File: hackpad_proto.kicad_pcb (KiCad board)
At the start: 2 copper layers, 110 x 97 mm, 40 parts, among them J1 Conn_01x04, SW1 SW_Push, SW10 SW_Push, SW11 SW_Push, SW12 SW_Push, SW13 RotaryEncoder_Switch, SW2 SW_Push, SW3 SW_Push, SW4 SW_Push, SW5 SW_Push, SW6 SW_Push, SW7 SW_Push, SW8 SW_Push, SW9 SW_Push, U1 XIAO-RP2040-DIP

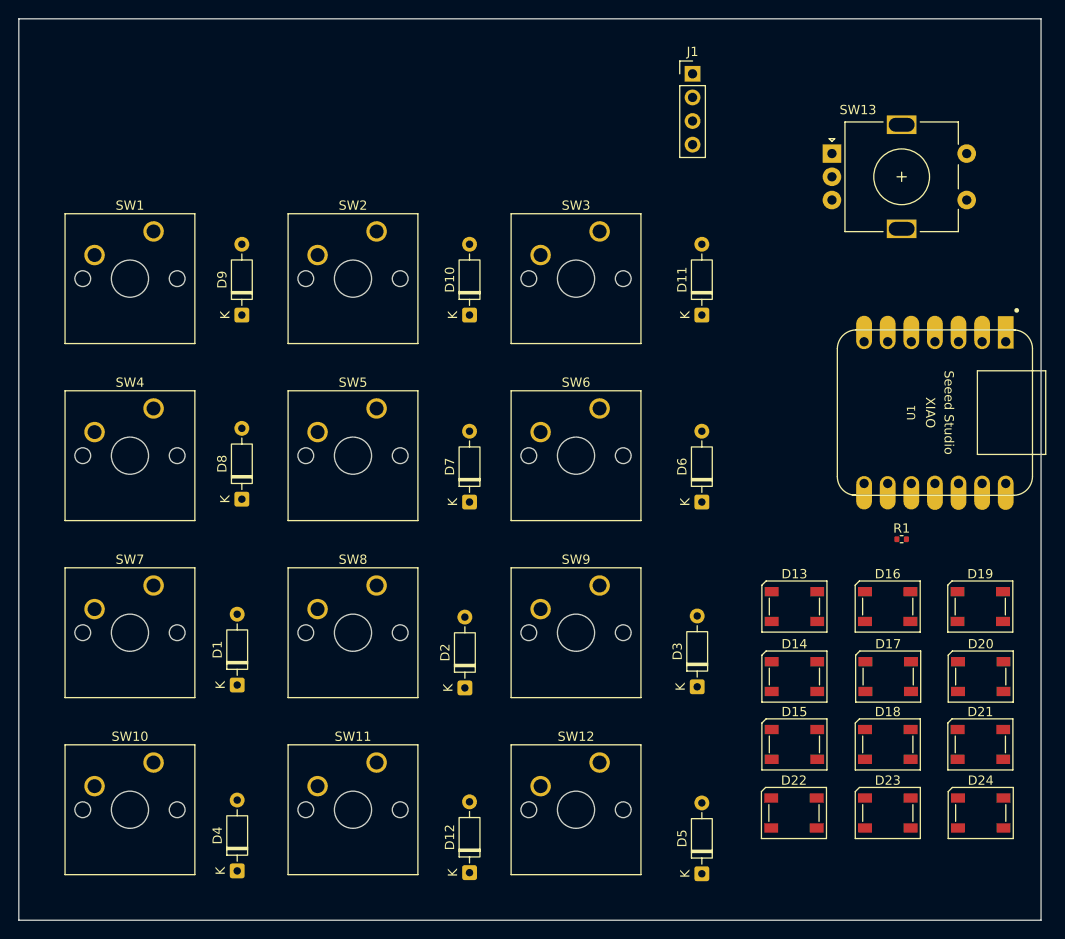
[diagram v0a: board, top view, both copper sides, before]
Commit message: Updated NostPad hardware design layout
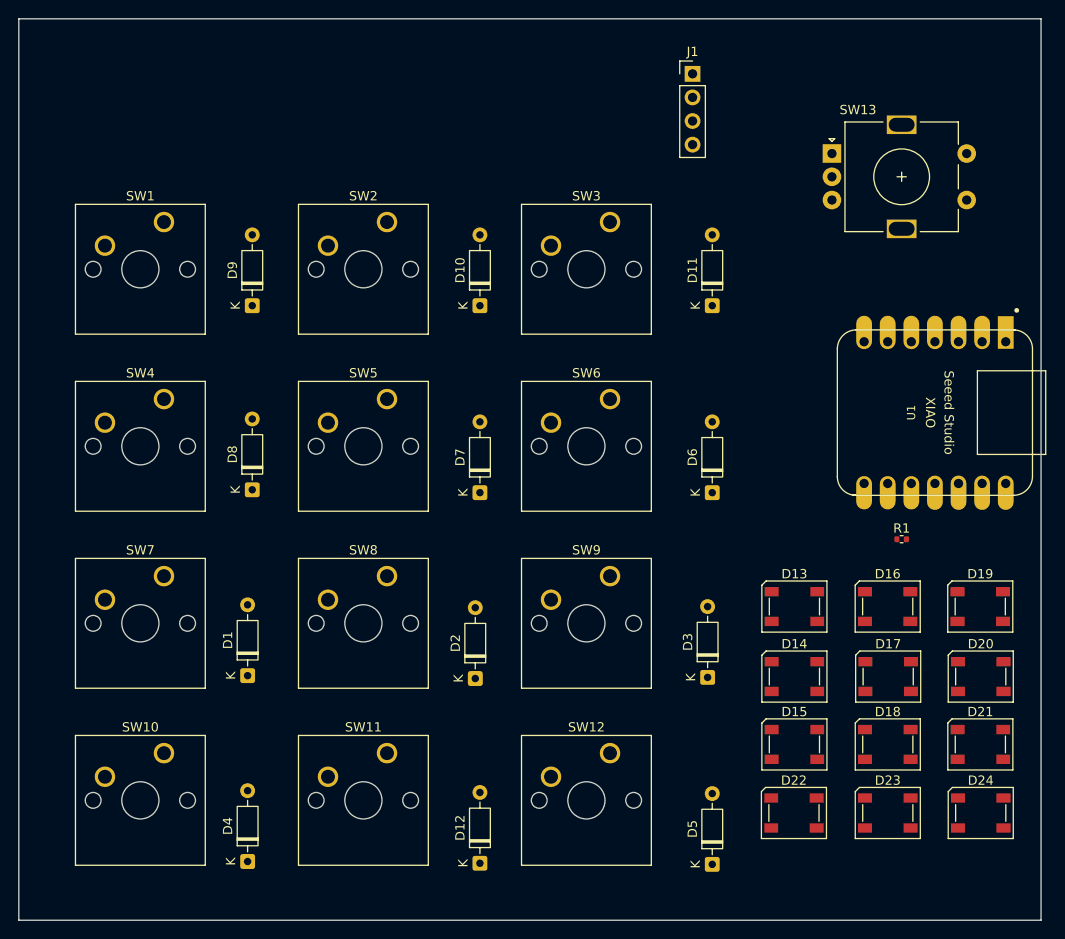
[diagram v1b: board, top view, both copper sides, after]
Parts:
- moved D2 1.51 mm to (70.1, 103.5)
- moved D5 1.51 mm to (95.6, 123.5)
- moved D6 1.51 mm to (95.6, 83.5)
- moved D7 1.51 mm to (70.6, 83.5)
- moved SW12 1.51 mm to (84.6, 111.5)
- moved SW3 1.51 mm to (84.6, 54.4)
- moved SW6 1.51 mm to (84.6, 73.4)
- moved SW9 1.51 mm to (84.6, 92.5)
- moved D10 1.51 mm to (70.6, 63.4)
- moved D11 1.51 mm to (95.6, 63.4)
- moved SW1 1.51 mm to (36.6, 54.4)
- moved SW10 1.51 mm to (36.6, 111.5)
- moved SW11 1.51 mm to (60.6, 111.5)
- moved SW2 1.51 mm to (60.6, 54.4)
- moved SW4 1.51 mm to (36.6, 73.4)
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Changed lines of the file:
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@@
 	(footprint "Button_Switch_Keyboard:SW_Cherry_MX_1.00u_PCB"
 		(layer "F.Cu")
-		(at 35.5 112.53)
+		(at 36.62 111.52)
 		(descr "Cherry MX keyswitch, 1.00u, PCB mount, http://cherryamericas.com/wp-content/uploads/2014/12/mx_cat.pdf")
 		(tags "Cherry MX keyswitch 1.00u PCB")
@@
 	(footprint "Button_Switch_Keyboard:SW_Cherry_MX_1.00u_PCB"
 		(layer "F.Cu")
-		(at 83.5 55.38)
+		(at 84.62 54.37)
 		(descr "Cherry MX keyswitch, 1.00u, PCB mount, http://cherryamericas.com/wp-content/uploads/2014/12/mx_cat.pdf")
 		(tags "Cherry MX keyswitch 1.00u PCB")
@@
 	(footprint "Diode_THT:D_DO-35_SOD27_P7.62mm_Horizontal"
 		(layer "F.Cu")
-		(at 69.5 84.5 90)
+		(at 70.62 83.49 90)
 		(descr "Diode, DO-35_SOD27 series, Axial, Horizontal, pin pitch=7.62mm, length*diameter=4*2mm^2, http://www.diodes.com/_files/packages/DO-35.pdf")
 		(tags "Diode DO-35_SOD27 series Axial Horizontal pin pitch 7.62mm  length 4mm diameter 2mm")
@@
 	(footprint "Button_Switch_Keyboard:SW_Cherry_MX_1.00u_PCB"
 		(layer "F.Cu")
-		(at 59.5 55.38)
+		(at 60.62 54.37)
 		(descr "Cherry MX keyswitch, 1.00u, PCB mount, http://cherryamericas.com/wp-content/uploads/2014/12/mx_cat.pdf")
 		(tags "Cherry MX keyswitch 1.00u PCB")
@@
 	(footprint "Diode_THT:D_DO-35_SOD27_P7.62mm_Horizontal"
 		(layer "F.Cu")
-		(at 45 64.38 90)
+		(at 46.12 63.37 90)
 		(descr "Diode, DO-35_SOD27 series, Axial, Horizontal, pin pitch=7.62mm, length*diameter=4*2mm^2, http://www.diodes.com/_files/packages/DO-35.pdf")
 		(tags "Diode DO-35_SOD27 series Axial Horizontal pin pitch 7.62mm  length 4mm diameter 2mm")
@@
 	(footprint "Diode_THT:D_DO-35_SOD27_P7.62mm_Horizontal"
 		(layer "F.Cu")
-		(at 94 104.38 90)
+		(at 95.12 103.37 90)
 		(descr "Diode, DO-35_SOD27 series, Axial, Horizontal, pin pitch=7.62mm, length*diameter=4*2mm^2, http://www.diodes.com/_files/packages/DO-35.pdf")
 		(tags "Diode DO-35_SOD27 series Axial Horizontal pin pitch 7.62mm  length 4mm diameter 2mm")
@@
 	(footprint "Button_Switch_Keyboard:SW_Cherry_MX_1.00u_PCB"
 		(layer "F.Cu")
-		(at 83.5 112.53)
+		(at 84.62 111.52)
 		(descr "Cherry MX keyswitch, 1.00u, PCB mount, http://cherryamericas.com/wp-content/uploads/2014/12/mx_cat.pdf")
 		(tags "Cherry MX keyswitch 1.00u PCB")
@@
 	(footprint "Diode_THT:D_DO-35_SOD27_P7.62mm_Horizontal"
 		(layer "F.Cu")
-		(at 69.5 124.38 90)
+		(at 70.62 123.37 90)
 		(descr "Diode, DO-35_SOD27 series, Axial, Horizontal, pin pitch=7.62mm, length*diameter=4*2mm^2, http://www.diodes.com/_files/packages/DO-35.pdf")
 		(tags "Diode DO-35_SOD27 series Axial Horizontal pin pitch 7.62mm  length 4mm diameter 2mm")
@@
 	(footprint "Button_Switch_Keyboard:SW_Cherry_MX_1.00u_PCB"
 		(layer "F.Cu")
-		(at 59.5 93.48)
+		(at 60.62 92.47)
 		(descr "Cherry MX keyswitch, 1.00u, PCB mount, http://cherryamericas.com/wp-content/uploads/2014/12/mx_cat.pdf")
 		(tags "Cherry MX keyswitch 1.00u PCB")
@@
 	(footprint "Button_Switch_Keyboard:SW_Cherry_MX_1.00u_PCB"
 		(layer "F.Cu")
-		(at 35.5 74.43)
+		(at 36.62 73.42)
 		(descr "Cherry MX keyswitch, 1.00u, PCB mount, http://cherryamericas.com/wp-content/uploads/2014/12/mx_cat.pdf")
 		(tags "Cherry MX keyswitch 1.00u PCB")
@@
 	(footprint "Diode_THT:D_DO-35_SOD27_P7.62mm_Horizontal"
 		(layer "F.Cu")
-		(at 94.5 64.38 90)
+		(at 95.62 63.37 90)
 		(descr "Diode, DO-35_SOD27 series, Axial, Horizontal, pin pitch=7.62mm, length*diameter=4*2mm^2, http://www.diodes.com/_files/packages/DO-35.pdf")
 		(tags "Diode DO-35_SOD27 series Axial Horizontal pin pitch 7.62mm  length 4mm diameter 2mm")
@@
 	(footprint "Button_Switch_Keyboard:SW_Cherry_MX_1.00u_PCB"
 		(layer "F.Cu")
-		(at 83.5 93.48)
+		(at 84.62 92.47)
 		(descr "Cherry MX keyswitch, 1.00u, PCB mount, http://cherryamericas.com/wp-content/uploads/2014/12/mx_cat.pdf")
 		(tags "Cherry MX keyswitch 1.00u PCB")
@@
 	(footprint "Button_Switch_Keyboard:SW_Cherry_MX_1.00u_PCB"
 		(layer "F.Cu")
-		(at 83.5 74.43)
+		(at 84.62 73.42)
 		(descr "Cherry MX keyswitch, 1.00u, PCB mount, http://cherryamericas.com/wp-content/uploads/2014/12/mx_cat.pdf")
 		(tags "Cherry MX keyswitch 1.00u PCB")
@@
 	(footprint "Diode_THT:D_DO-35_SOD27_P7.62mm_Horizontal"
 		(layer "F.Cu")
-		(at 69.5 64.38 90)
+		(at 70.62 63.37 90)
 		(descr "Diode, DO-35_SOD27 series, Axial, Horizontal, pin pitch=7.62mm, length*diameter=4*2mm^2, http://www.diodes.com/_files/packages/DO-35.pdf")
 		(tags "Diode DO-35_SOD27 series Axial Horizontal pin pitch 7.62mm  length 4mm diameter 2mm")
@@
 	(footprint "Diode_THT:D_DO-35_SOD27_P7.62mm_Horizontal"
 		(layer "F.Cu")
-		(at 44.5 124.19 90)
+		(at 45.62 123.18 90)
 		(descr "Diode, DO-35_SOD27 series, Axial, Horizontal, pin pitch=7.62mm, length*diameter=4*2mm^2, http://www.diodes.com/_files/packages/DO-35.pdf")
 		(tags "Diode DO-35_SOD27 series Axial Horizontal pin pitch 7.62mm  length 4mm diameter 2mm")
@@
 	(footprint "Diode_THT:D_DO-35_SOD27_P7.62mm_Horizontal"
 		(layer "F.Cu")
-		(at 44.5 104.19 90)
+		(at 45.62 103.18 90)
 		(descr "Diode, DO-35_SOD27 series, Axial, Horizontal, pin pitch=7.62mm, length*diameter=4*2mm^2, http://www.diodes.com/_files/packages/DO-35.pdf")
 		(tags "Diode DO-35_SOD27 series Axial Horizontal pin pitch 7.62mm  length 4mm diameter 2mm")
@@
 	(footprint "Button_Switch_Keyboard:SW_Cherry_MX_1.00u_PCB"
 		(layer "F.Cu")
-		(at 59.5 112.53)
+		(at 60.62 111.52)
 		(descr "Cherry MX keyswitch, 1.00u, PCB mount, http://cherryamericas.com/wp-content/uploads/2014/12/mx_cat.pdf")
 		(tags "Cherry MX keyswitch 1.00u PCB")
@@
 	(footprint "Diode_THT:D_DO-35_SOD27_P7.62mm_Horizontal"
 		(layer "F.Cu")
-		(at 69 104.5 90)
+		(at 70.12 103.49 90)
 		(descr "Diode, DO-35_SOD27 series, Axial, Horizontal, pin pitch=7.62mm, length*diameter=4*2mm^2, http://www.diodes.com/_files/packages/DO-35.pdf")
 		(tags "Diode DO-35_SOD27 series Axial Horizontal pin pitch 7.62mm  length 4mm diameter 2mm")
@@
 	(footprint "Button_Switch_Keyboard:SW_Cherry_MX_1.00u_PCB"
 		(layer "F.Cu")
-		(at 59.5 74.43)
+		(at 60.62 73.42)
 		(descr "Cherry MX keyswitch, 1.00u, PCB mount, http://cherryamericas.com/wp-content/uploads/2014/12/mx_cat.pdf")
 		(tags "Cherry MX keyswitch 1.00u PCB")
@@
 	(footprint "Diode_THT:D_DO-35_SOD27_P7.62mm_Horizontal"
 		(layer "F.Cu")
-		(at 94.5 84.5 90)
+		(at 95.62 83.49 90)
 		(descr "Diode, DO-35_SOD27 series, Axial, Horizontal, pin pitch=7.62mm, length*diameter=4*2mm^2, http://www.diodes.com/_files/packages/DO-35.pdf")
 		(tags "Diode DO-35_SOD27 series Axial Horizontal pin pitch 7.62mm  length 4mm diameter 2mm")
@@
 	(footprint "Button_Switch_Keyboard:SW_Cherry_MX_1.00u_PCB"
 		(layer "F.Cu")
-		(at 35.5 55.38)
+		(at 36.62 54.37)
 		(descr "Cherry MX keyswitch, 1.00u, PCB mount, http://cherryamericas.com/wp-content/uploads/2014/12/mx_cat.pdf")
 		(tags "Cherry MX keyswitch 1.00u PCB")
@@
 	(footprint "Diode_THT:D_DO-35_SOD27_P7.62mm_Horizontal"
 		(layer "F.Cu")
-		(at 45 84.19 90)
+		(at 46.12 83.18 90)
 		(descr "Diode, DO-35_SOD27 series, Axial, Horizontal, pin pitch=7.62mm, length*diameter=4*2mm^2, http://www.diodes.com/_files/packages/DO-35.pdf")
 		(tags "Diode DO-35_SOD27 series Axial Horizontal pin pitch 7.62mm  length 4mm diameter 2mm")
@@
 	(footprint "Diode_THT:D_DO-35_SOD27_P7.62mm_Horizontal"
 		(layer "F.Cu")
-		(at 94.5 124.5 90)
+		(at 95.62 123.49 90)
 		(descr "Diode, DO-35_SOD27 series, Axial, Horizontal, pin pitch=7.62mm, length*diameter=4*2mm^2, http://www.diodes.com/_files/packages/DO-35.pdf")
 		(tags "Diode DO-35_SOD27 series Axial Horizontal pin pitch 7.62mm  length 4mm diameter 2mm")
@@
 	(footprint "Button_Switch_Keyboard:SW_Cherry_MX_1.00u_PCB"
 		(layer "F.Cu")
-		(at 35.5 93.48)
+		(at 36.62 92.47)
 		(descr "Cherry MX keyswitch, 1.00u, PCB mount, http://cherryamericas.com/wp-content/uploads/2014/12/mx_cat.pdf")
 		(tags "Cherry MX keyswitch 1.00u PCB")
